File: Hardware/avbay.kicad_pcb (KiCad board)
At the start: 2 copper layers, 45.7 x 95.3 mm, 53 parts, among them P1 TERM_BLOCK_2.54MM_2POS, P2 CONN_6, P3 TERM_BLOCK_2.54MM_8POS, P4 TERM_BLOCK_2.54MM_5POS, P5 TERM_BLOCK_2.54MM_5POS, P6 TERM_BLOCK_2.54MM_2POS, P7 TERM_BLOCK_2.54MM_8POS, Q1 DMN2041LSD, Q2 BSS138DW, Q3 DMN2041LSD, Q4 BSS138DW, SW2 SW_PUSH, SW3 SW_PUSH, U1 STM32F411RE_LQFP64, U2 LM1084IS-3.3/NOPB, U3 LM1084IS-5.0/NOPB, U4 MS5611, U5 HMC5883L, U6 L3G4200D

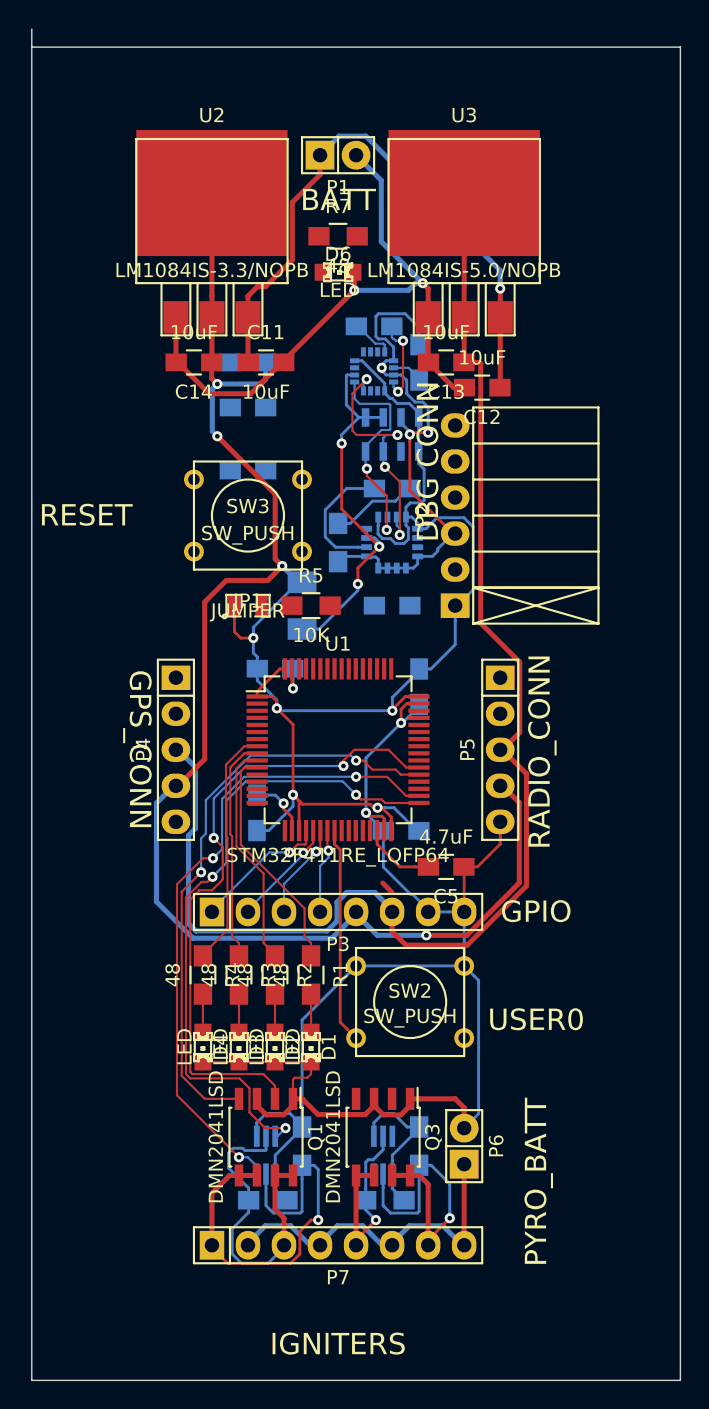
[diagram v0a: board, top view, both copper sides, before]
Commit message: Finished routing.
Board awaiting review
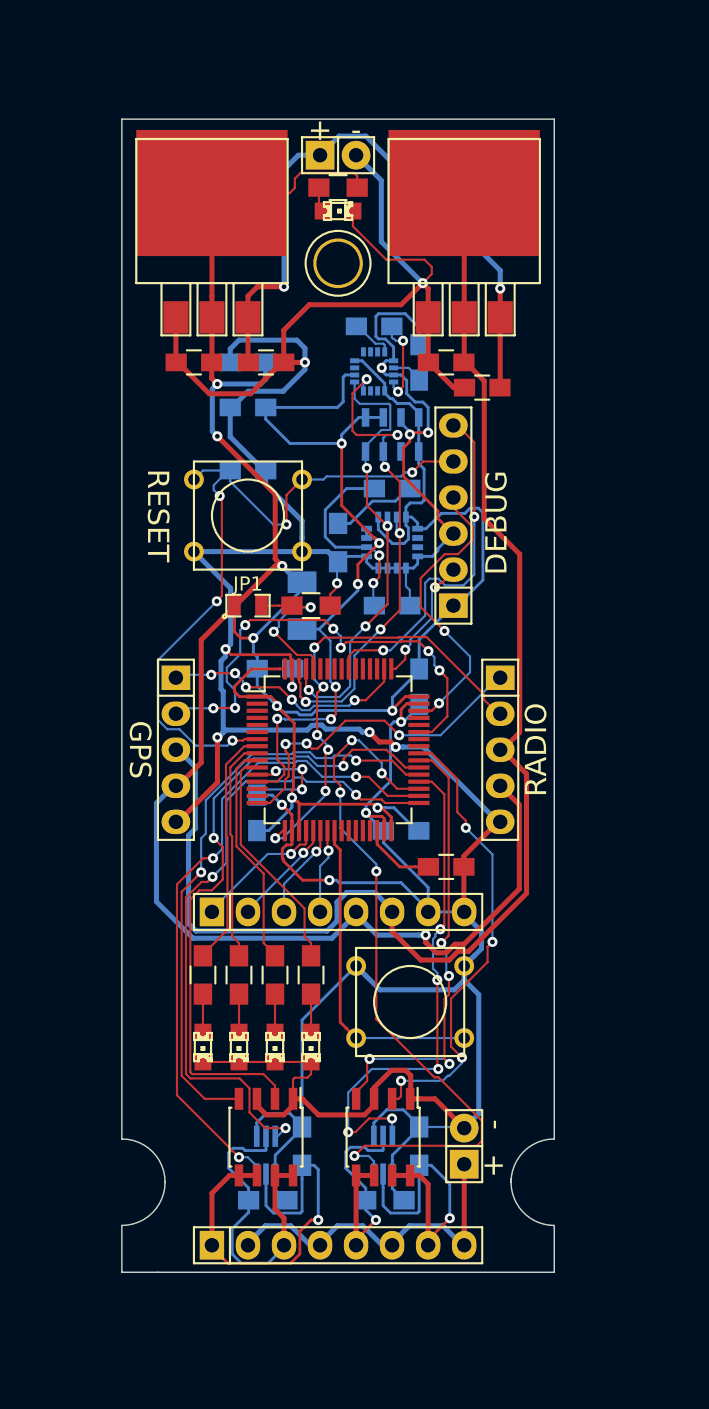
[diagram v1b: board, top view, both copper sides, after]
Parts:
- added 1pin: VAL**, Connect:1pin, F.Cu at (152.4, 53.3)
- P2: footprint Socket_Strips:Socket_Strip_Angled_1x06 -> Socket_Strips:Socket_Strip_Straight_1x06
- moved D6 4.32 mm to (152.4, 49.7)
- moved R7 3.43 mm to (152.4, 48.0)
- moved P2 0.13 mm to (160.5, 71.1)
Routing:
- net GND: track 215.6 -> 349.2 mm, vias 9 -> 18
- net /MCU/NRST: track 0.00 -> 51.9 mm, vias 0 -> 5
- net /MCU/SENSE3: track 0.00 -> 51.7 mm, vias 0 -> 5
- net /MCU/SENSE4: track 0.00 -> 36.6 mm, vias 0 -> 5
- net /MCU/USART_RX: track 0.00 -> 33.4 mm, vias 0 -> 7
- net /MCU/RADIO_RX: track 0.00 -> 32.8 mm, vias 0 -> 6
- net /MCU/TRIGGER4: track 0.00 -> 32.6 mm, vias 0 -> 4
- net /MCU/TRIGGER3: track 0.00 -> 32.5 mm, vias 0 -> 4
- net /MCU/VDDA: track 27.1 -> 56.3 mm, vias 3 -> 6
- net /MCU/JTDO-SWO: track 0.00 -> 25.0 mm, vias 0 -> 2
- net /MCU/RADIO_TX: track 0.00 -> 23.9 mm, vias 0 -> 3
- net /MCU/JTMS-SWDIO: track 0.00 -> 21.1 mm, vias 0 -> 2
- net 3V3: track 199.1 -> 220.0 mm
- net /Sensors/SDA: track 18.0 -> 36.4 mm, vias 4 -> 6
- net /Sensors/SCL: track 15.3 -> 33.1 mm, vias 2 -> 4
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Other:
- board size 45.7 x 95.3 mm -> 30.5 x 81.3 mm
- board text added: "+"
- board text added: "-"
- board text added: "DEBUG"
- board text added: "GPS"
- board text added: "RADIO"
- board text removed: "BATT"
- board text removed: "DBG CONN"
- board text removed: "GPIO"
- board text removed: "GPS_CONN"
- board text removed: "IGNITERS"
- board text removed: "PYRO_BATT"
- board text removed: "RADIO_CONN"
- board text removed: "USER0"
